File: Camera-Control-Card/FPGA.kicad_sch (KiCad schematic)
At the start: 63 parts, among them U1 LCMXO2-7000HC-6TG144I, U11 T602-025.0M

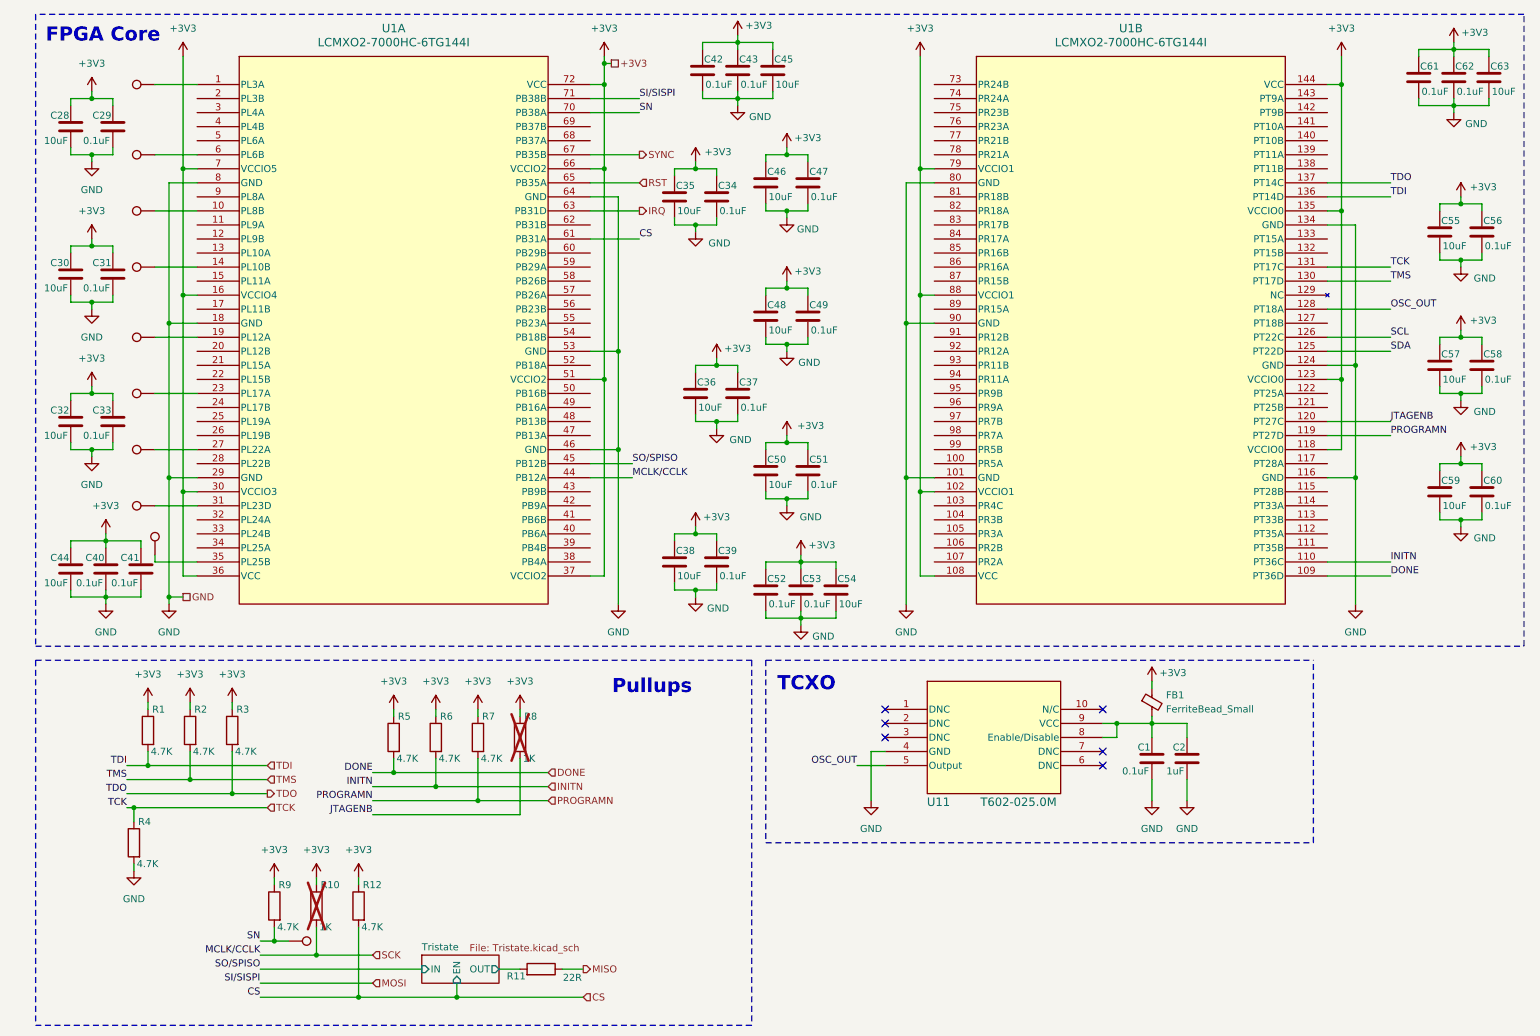
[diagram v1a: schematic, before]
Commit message: test
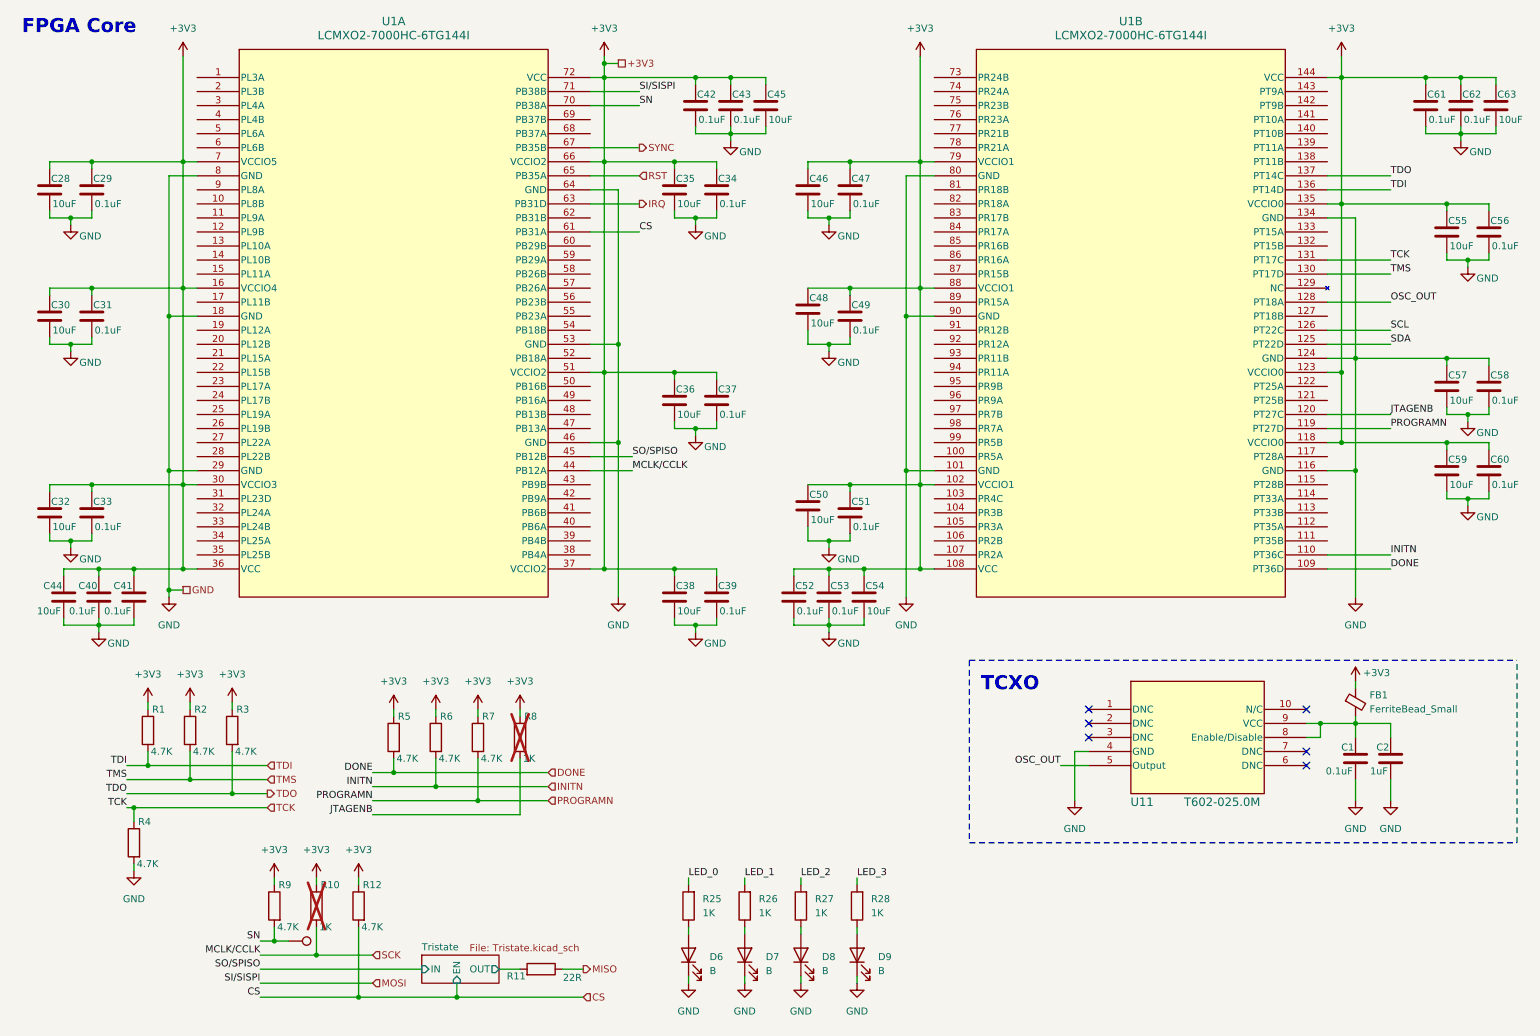
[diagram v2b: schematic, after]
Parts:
- removed TP10, TP11, TP12, TP13, TP14, TP15, TP7, TP8, TP9: TestPoint, TestPoint:TestPoint_Pad_1.0x1.0mm, symbol Connector:TestPoint
- added D6, D7, D8, D9: B, Resistor_SMD:R_0603_1608Metric, symbol Device:LED
- added R25, R26, R27, R28: 1K, Resistor_SMD:R_0603_1608Metric, symbol Device:R
- C1, C2: footprint Capacitor_SMD:C_0805_2012Metric -> Capacitor_SMD:C_0603_1608Metric
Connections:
- net +3V3: no longer C57.1, C58.1
- net GND: now also C57.1, C58.1, D6.1 (K), D7.1 (K), D8.1 (K), D9.1 (K)
- new net: D9.2 (A), R28.1
- new net: D7.2 (A), R26.1
- new net: D8.2 (A), R27.1
- new net: D6.2 (A), R25.1
- new net LED_0: R25.2
- new net LED_1: R26.2
- new net LED_2: R27.2
- new net LED_3: R28.2
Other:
- note removed: "Pullups"
- moved on the sheet: C1, C2, C28, C29, C30, C31, C32, C33, C34, C35, C36, C37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
